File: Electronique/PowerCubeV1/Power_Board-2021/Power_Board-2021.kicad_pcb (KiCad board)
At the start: 2 copper layers, 95.2 x 95.2 mm, 118 parts, among them J1 Conn_01x02_Male, J1001 Conn_02x20_Odd_Even, J1002 Conn_02x20_Odd_Even, Q2001 IRLL3303, Q2002 IRLL3303, Q2003 IRLL3303, Q2004 IRLL3303, SW1 SW_SPST, U1 BTS50055-1TMA, U2 MCP3427-xUN, U2001 L5973D, U2002 L5973D, U2003 L5973D, U2004 L5973D, U3 MCP3428

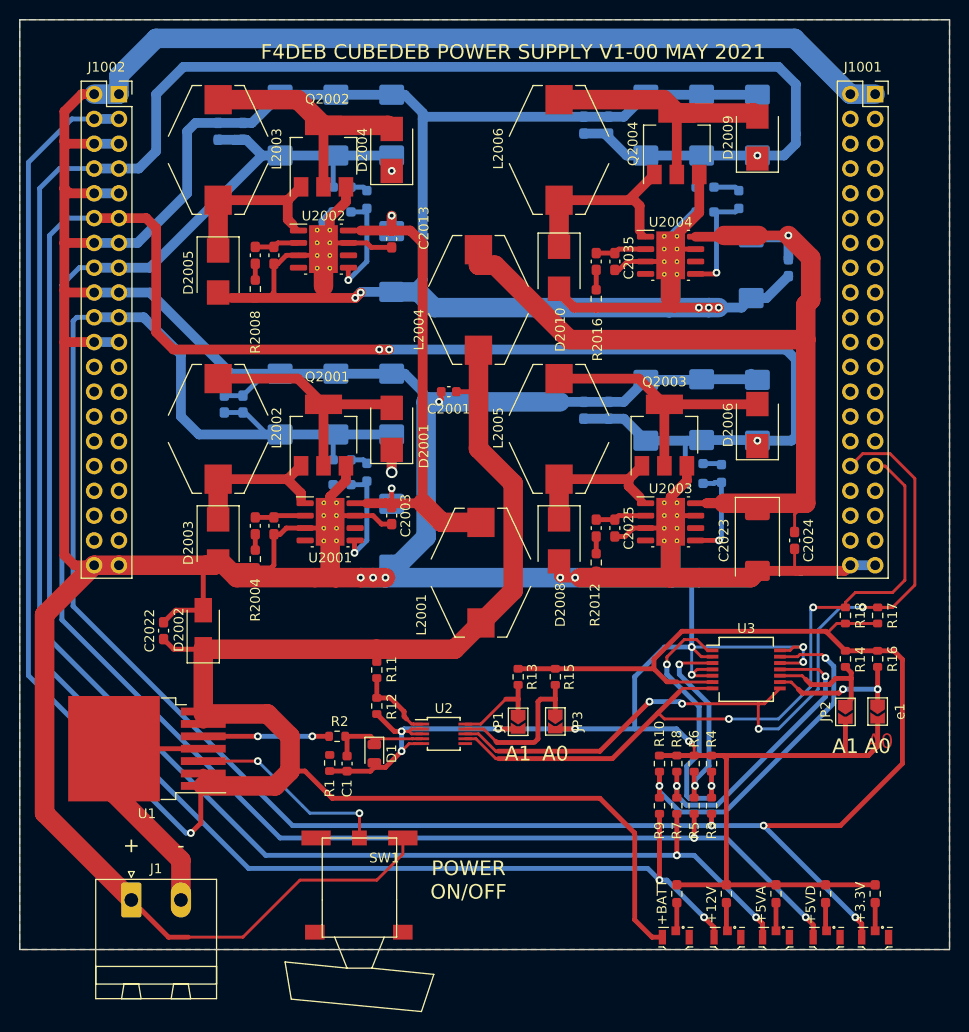
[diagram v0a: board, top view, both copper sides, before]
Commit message: CPU
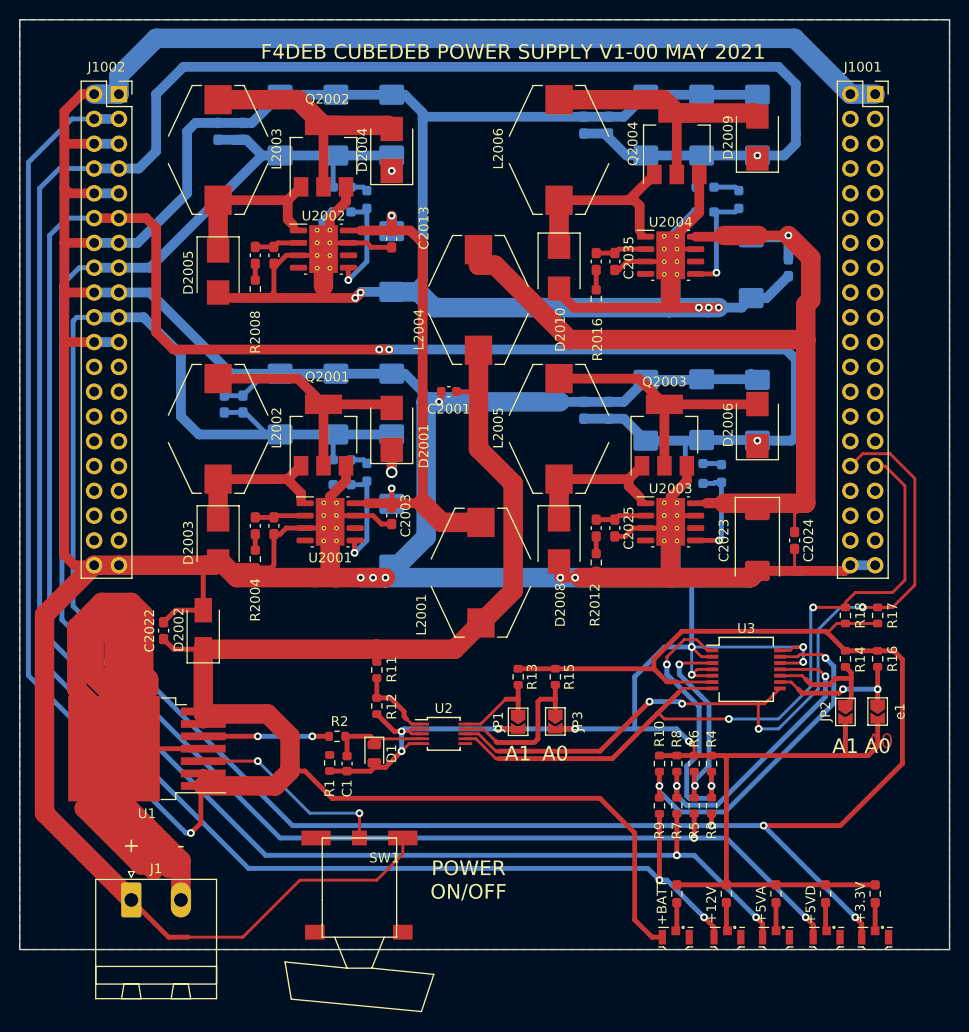
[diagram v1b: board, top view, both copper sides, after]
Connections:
- SW1 pad 4: (no net) -> GND
- SW1 pad 5: (no net) -> GND
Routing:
- net +VSW: track 27.5 -> 120.1 mm
